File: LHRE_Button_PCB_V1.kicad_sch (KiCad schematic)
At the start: 28 parts, among them J1 Conn_01x12_Female, J2 Conn_01x12_Female, J4 Conn_01x02_Female, SW1 Dashboard_Button, SW2 Dashboard_Button, SW3 Dashboard_Button, SW4 Dashboard_Button, SW5 Dashboard_Button, SW6 Dashboard_Button

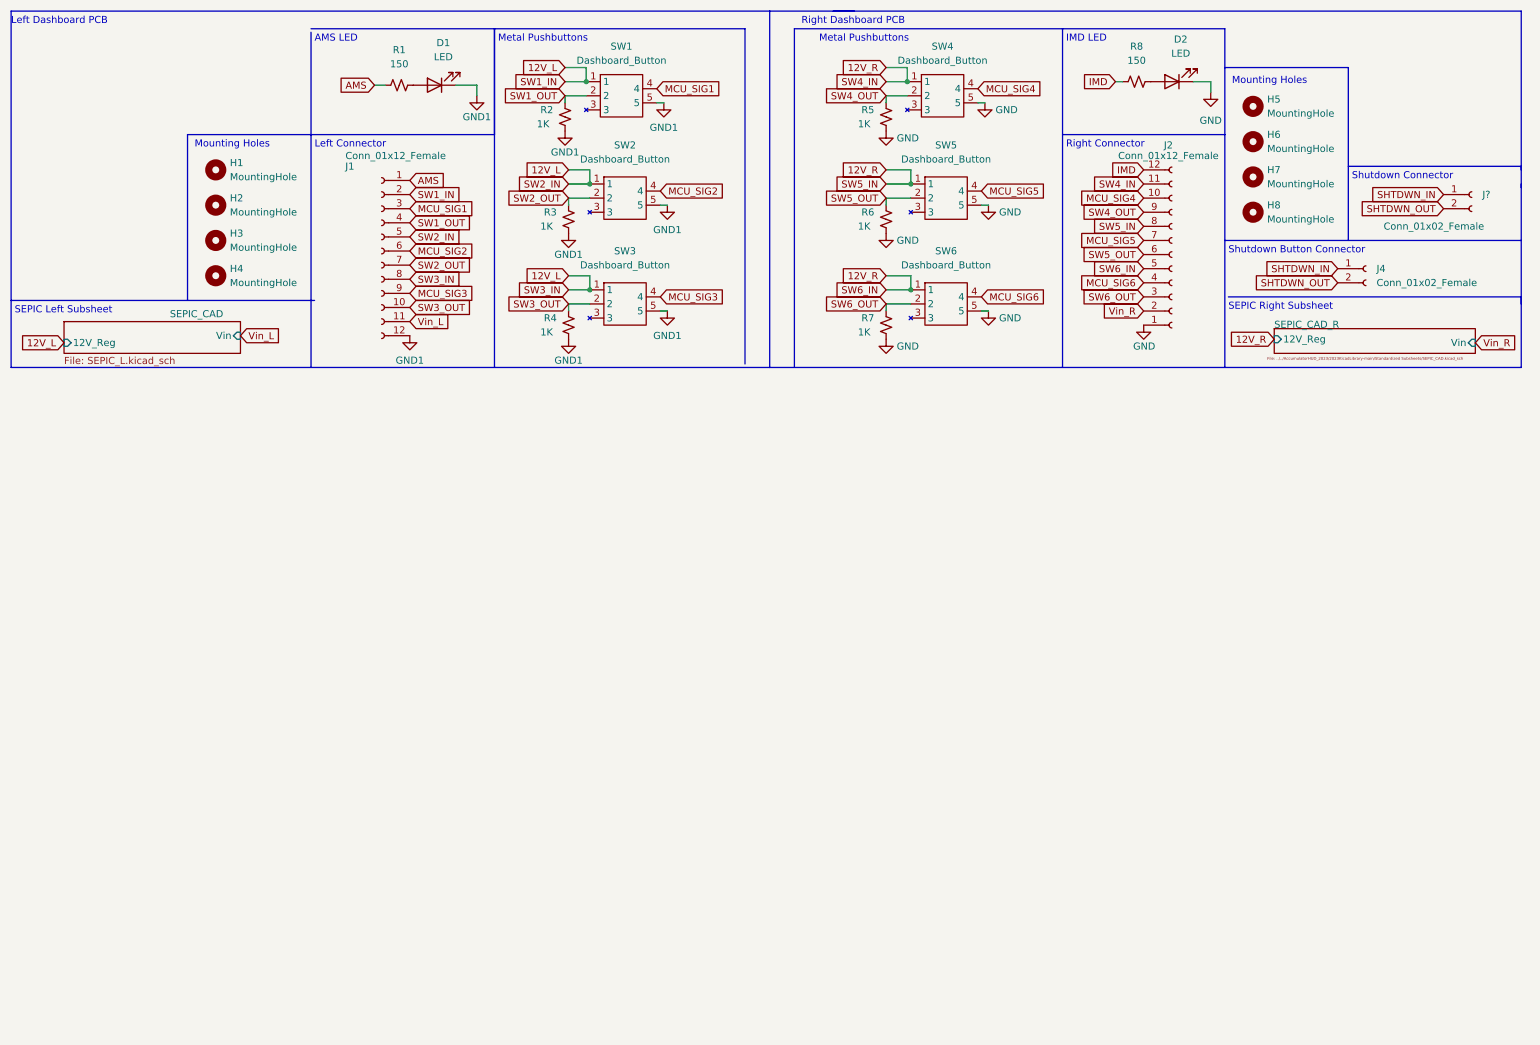
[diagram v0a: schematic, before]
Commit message: REV2
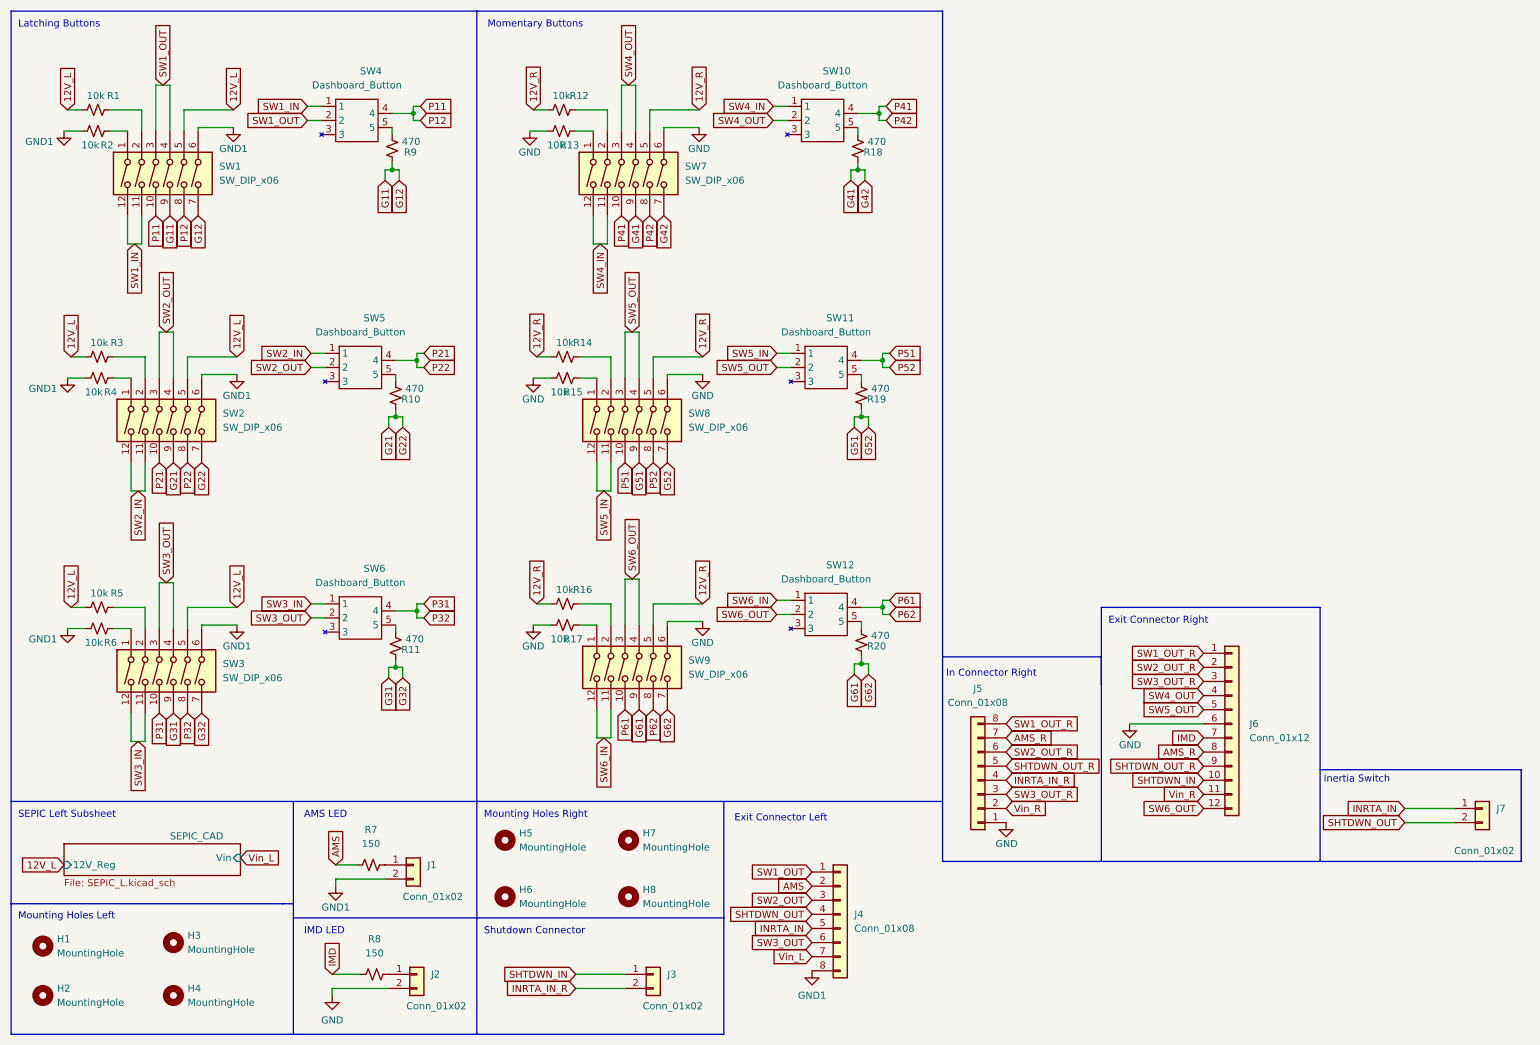
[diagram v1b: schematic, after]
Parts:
- removed D1, D2: LED, Dashboard_LED:LEDC1608X80N, symbol Device:LED
- removed J1, J2: Conn_01x12_Female, Connector_Molex:Molex_Micro-Fit_3.0_43650-1210_1x12-1MP_P3.00mm_Horizontal, symbol Connector:Conn_01x12_Female
- removed J4: Conn_01x02_Female, Connector_Molex:Molex_Micro-Fit_3.0_43650-0210_1x02-1MP_P3.00mm_Horizontal, symbol Connector:Conn_01x02_Female
- removed J?: Conn_01x02_Female, Connector_Wire:SolderWire-0.5sqmm_1x02_P4.8mm_D0.9mm_OD2.3mm, symbol Connector:Conn_01x02_Female
- removed R7: 1K, Resistor_SMD:R_0603_1608Metric, symbol Device:R_Small_US
- removed SW2, SW3, SW4: Dashboard_Button, Dashboard_LED:Dashboard_Btn, symbol Dashboard:Dashboard_Button
- added J1, J2, J3, J7: Conn_01x02, Connector_Molex:Molex_Micro-Fit_3.0_43650-0215_1x02_P3.00mm_Vertical, symbol Connector_Generic:Conn_01x02
- added J4, J5: Conn_01x08, Connector_Molex:Molex_Micro-Fit_3.0_43650-0800_1x08_P3.00mm_Horizontal, symbol Connector_Generic:Conn_01x08
- added J6: Conn_01x12, Connector_Molex:Molex_Micro-Fit_3.0_43045-1212_2x06_P3.00mm_Vertical, symbol Connector_Generic:Conn_01x12
- added R1, R12, R13, R14, R15, R16, R17: 10k, Resistor_SMD:R_0603_1608Metric, symbol Device:R_Small_US
- added R10, R11, R18, R19, R20, R9: 470, Resistor_SMD:R_0603_1608Metric, symbol Device:R_Small_US
- added SW1, SW2, SW3, SW7, SW8, SW9: SW_DIP_x06, Through_DIP_6:18253604, symbol Switch:SW_DIP_x06
- added SW10, SW11, SW12: Dashboard_Button, Dashboard_LED:Dashboard_Btn, symbol Dashboard:Dashboard_Button
- R2, R3, R4, R5, R6: value 1K -> 10k
- renumbered R1 to R7, SW1 to SW4
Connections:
- net 12V_L: now also R3.1, R5.1, R1.1, SW1.5, SW2.5, SW3.5; no longer SW4.1
- net 12V_R: now also R12.1, R14.1, R16.1, SW7.5, SW8.5, SW9.5; no longer SW5.1, SW6.1
- net AMS: now also J4.2 (Pin_2)
- net GND: now also J2.2 (Pin_2), J5.1 (Pin_1), J6.6 (Pin_6), R13.1, R15.1, R17.1, SW7.6, SW8.6, SW9.6; no longer R5.1, R6.1, SW5.5, SW6.5
- net GND1: now also R6.1, J1.2 (Pin_2), J4.8 (Pin_8), SW1.6, SW2.6, SW3.6; no longer R3.1, SW4.5
- net IMD: now also J6.7 (Pin_7)
- net SHTDWN_IN: now also J3.1 (Pin_1), J6.10 (Pin_10)
- net SHTDWN_OUT: now also J4.4 (Pin_4), J7.2 (Pin_2)
- net SW1_OUT: now also J4.1 (Pin_1), SW1.3, SW1.4; no longer R2.2
- net SW2_OUT: now also SW5.2, J4.3 (Pin_3), SW2.3, SW2.4; no longer R3.2
- net SW3_OUT: now also SW6.2, J4.6 (Pin_6), SW3.3, SW3.4; no longer R4.2
- net SW4_OUT: now also J6.4 (Pin_4), SW10.2, SW7.3, SW7.4; no longer R5.2
- net SW5_OUT: now also J6.5 (Pin_5), SW11.2, SW8.3, SW8.4; no longer R6.2, SW5.2
- net SW6_OUT: now also J6.12 (Pin_12), SW12.2, SW9.3, SW9.4; no longer SW6.2
- net Vin_L: now also J4.7 (Pin_7)
- net Vin_R: now also J5.2 (Pin_2), J6.11 (Pin_11)
- net at R8.2: now also J2.1 (Pin_1)
- net at R7.2: now also J1.1 (Pin_1)
- net MCU_SIG1 renamed P11
- net P11: now also SW1.10, SW1.8
- net MCU_SIG5 renamed P21
- net P21: now also SW2.10, SW2.8
- net MCU_SIG6 renamed P31
- net P31: now also SW3.10, SW3.8
- new net: R11.2, SW6.5
- new net: R19.2, SW11.5
- new net: R5.2, SW3.2
- new net: R15.2, SW8.1
- new net: R18.2, SW10.5
- new net: R10.2, SW5.5
- new net: R17.2, SW9.1
- new net: R4.2, SW2.1
- new net: R3.2, SW2.2
- new net: R16.2, SW9.2
- new net: R9.2, SW4.5
- new net: R6.2, SW3.1
- new net: R20.2, SW12.5
- new net: R14.2, SW8.2
- new net: R13.2, SW7.1
- new net: R1.2, SW1.2
- new net: R12.2, SW7.2
- new net: R2.2, SW1.1
- new net AMS_R: J5.7 (Pin_7), J6.8 (Pin_8)
- new net G11: R9.1, SW1.7, SW1.9
- new net G21: R10.1, SW2.7, SW2.9
- new net G31: R11.1, SW3.7, SW3.9
- new net G41: R18.1, SW7.7, SW7.9
- new net G51: R19.1, SW8.7, SW8.9
- new net G61: R20.1, SW9.7, SW9.9
- new net INRTA_IN: J4.5 (Pin_5), J7.1 (Pin_1)
- new net INRTA_IN_R: J3.2 (Pin_2), J5.4 (Pin_4)
- new net P41: SW10.4, SW7.10, SW7.8
- new net P51: SW11.4, SW8.10, SW8.8
- new net P61: SW12.4, SW9.10, SW9.8
- new net SHTDWN_OUT_R: J5.5 (Pin_5), J6.9 (Pin_9)
- new net SW1_IN: SW1.11, SW1.12, SW4.1
- new net SW1_OUT_R: J5.8 (Pin_8), J6.1 (Pin_1)
- new net SW2_IN: SW2.11, SW2.12, SW5.1
- new net SW2_OUT_R: J5.6 (Pin_6), J6.2 (Pin_2)
- new net SW3_IN: SW3.11, SW3.12, SW6.1
- new net SW3_OUT_R: J5.3 (Pin_3), J6.3 (Pin_3)
- new net SW4_IN: SW10.1, SW7.11, SW7.12
- new net SW5_IN: SW11.1, SW8.11, SW8.12
- new net SW6_IN: SW12.1, SW9.11, SW9.12
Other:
- removed sheet SEPIC_CAD_R
- note added: "Exit Connector Left"
- note added: "Exit Connector Right"
- note added: "In Connector Right"
- note added: "Inertia Switch"
- note added: "Latching Buttons"
- note added: "Momentary Buttons"
- note added: "Mounting Holes Left"
- note added: "Mounting Holes Right"
- note removed: "Left Connector"
- note removed: "Left Dashboard PCB"
- note removed: "Metal Pushbuttons"
- note removed: "Mounting Holes"
- note removed: "Right Connector"
- note removed: "Right Dashboard PCB"
- note removed: "SEPIC Right Subsheet"
- note removed: "Shutdown Button Connector"
- moved on the sheet: H1, H2, H3, H4, H5, H6, H7, H8, R7, R8, SW4
